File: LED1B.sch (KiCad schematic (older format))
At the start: 18 parts

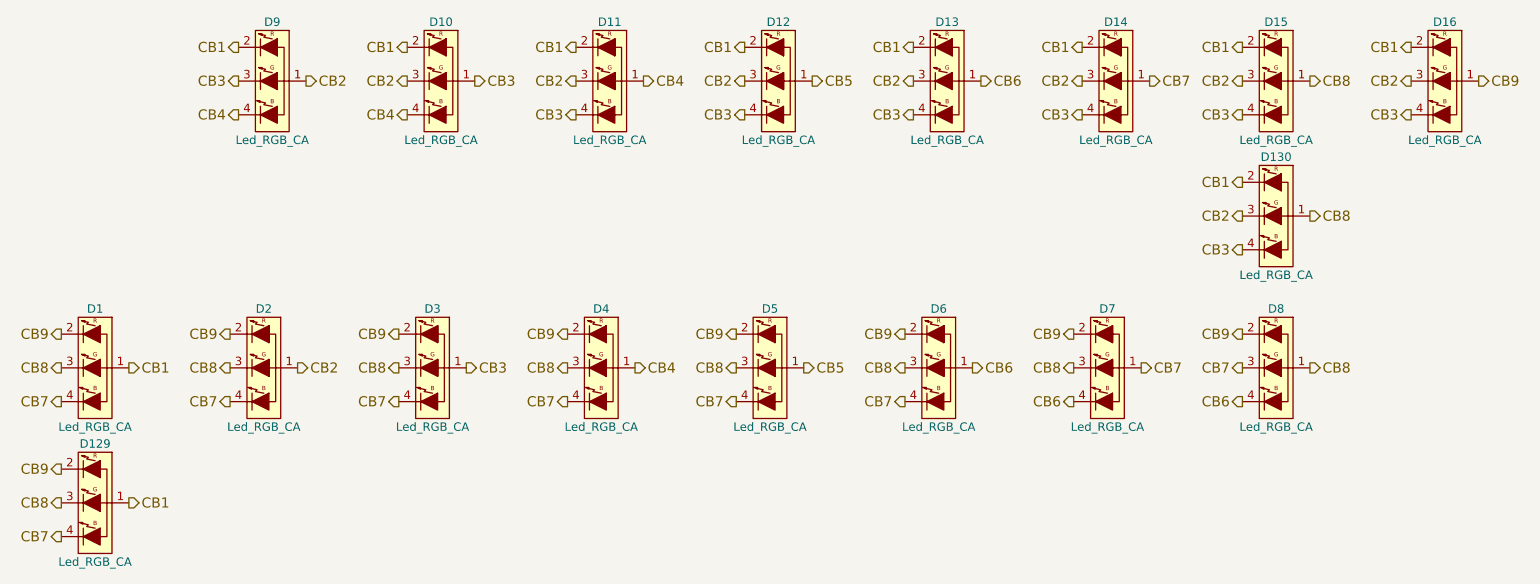
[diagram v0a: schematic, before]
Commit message: Did some visual cleanup.
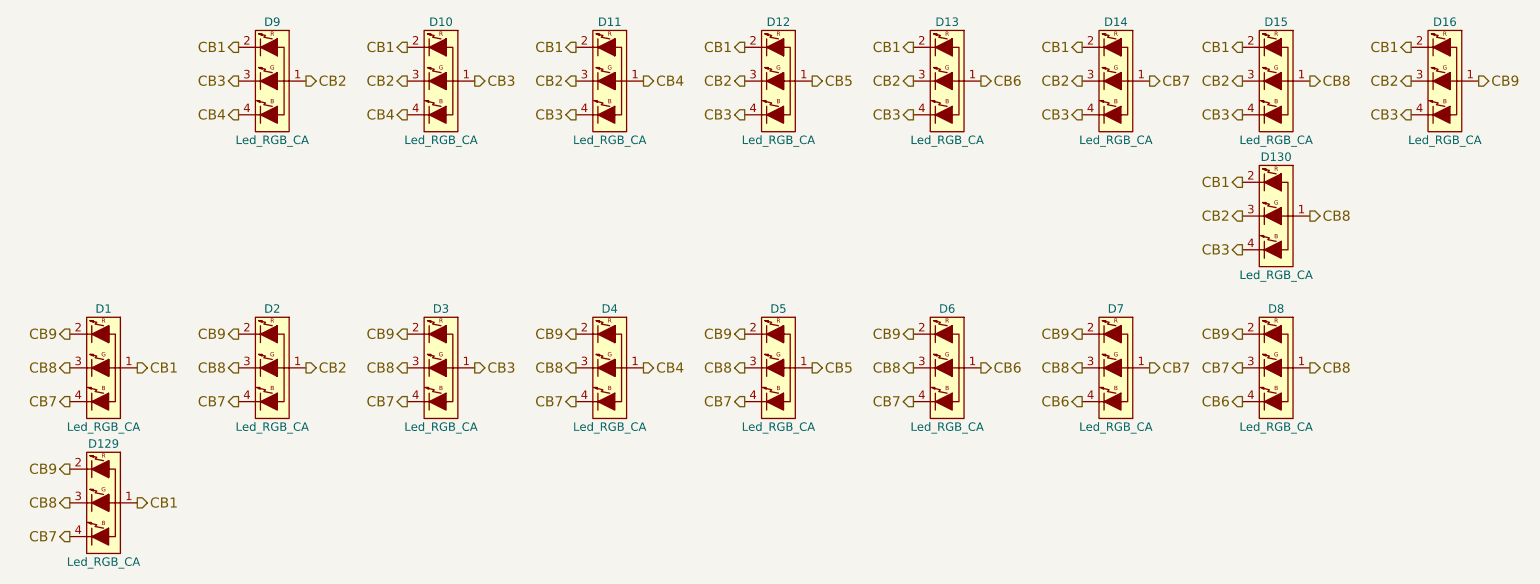
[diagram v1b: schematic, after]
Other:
- moved on the sheet: D1, D129, D2, D3, D4, D5, D6, D7
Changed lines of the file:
@@
 $Descr A4 11693 8268
 encoding utf-8
-Sheet 2 6
+Sheet 4 6
 Title ""
 Date ""
@@
 L Led_RGB_CA D1
 U 1 1 56C0E01C
-P 1950 3450
-F 0 "D1" H 1950 3800 50  0000 C CNN
-F 1 "Led_RGB_CA" H 1950 3100 50  0000 C CNN
-F 2 "mx2a:RGB" H 1905 3400 50  0001 C CNN
-F 3 "" H 1905 3400 50  0000 C CNN
-	1    1950 3450
+P 2000 3450
+F 0 "D1" H 2000 3800 50  0000 C CNN
+F 1 "Led_RGB_CA" H 2000 3100 50  0000 C CNN
+F 2 "mx2a:RGB" H 1955 3400 50  0001 C CNN
+F 3 "" H 1955 3400 50  0000 C CNN
+	1    2000 3450
 	1    0    0    -1
 $EndComp
@@
 L Led_RGB_CA D2
 U 1 1 56C0EC82
-P 2950 3450
-F 0 "D2" H 2950 3800 50  0000 C CNN
-F 1 "Led_RGB_CA" H 2950 3100 50  0000 C CNN
-F 2 "mx2a:RGB" H 2905 3400 50  0001 C CNN
-F 3 "" H 2905 3400 50  0000 C CNN
-	1    2950 3450
+P 3000 3450
+F 0 "D2" H 3000 3800 50  0000 C CNN
+F 1 "Led_RGB_CA" H 3000 3100 50  0000 C CNN
+F 2 "mx2a:RGB" H 2955 3400 50  0001 C CNN
+F 3 "" H 2955 3400 50  0000 C CNN
+	1    3000 3450
 	1    0    0    -1
 $EndComp
@@
 L Led_RGB_CA D3
 U 1 1 56C0F4C6
-P 3950 3450
-F 0 "D3" H 3950 3800 50  0000 C CNN
-F 1 "Led_RGB_CA" H 3950 3100 50  0000 C CNN
-F 2 "mx2a:RGB" H 3905 3400 50  0001 C CNN
-F 3 "" H 3905 3400 50  0000 C CNN
-	1    3950 3450
+P 4000 3450
+F 0 "D3" H 4000 3800 50  0000 C CNN
+F 1 "Led_RGB_CA" H 4000 3100 50  0000 C CNN
+F 2 "mx2a:RGB" H 3955 3400 50  0001 C CNN
+F 3 "" H 3955 3400 50  0000 C CNN
+	1    4000 3450
 	1    0    0    -1
 $EndComp
@@
 L Led_RGB_CA D4
 U 1 1 56C1065D
-P 4950 3450
-F 0 "D4" H 4950 3800 50  0000 C CNN
-F 1 "Led_RGB_CA" H 4950 3100 50  0000 C CNN
-F 2 "mx2a:RGB" H 4905 3400 50  0001 C CNN
-F 3 "" H 4905 3400 50  0000 C CNN
-	1    4950 3450
+P 5000 3450
+F 0 "D4" H 5000 3800 50  0000 C CNN
+F 1 "Led_RGB_CA" H 5000 3100 50  0000 C CNN
+F 2 "mx2a:RGB" H 4955 3400 50  0001 C CNN
+F 3 "" H 4955 3400 50  0000 C CNN
+	1    5000 3450
 	1    0    0    -1
 $EndComp
@@
 L Led_RGB_CA D5
 U 1 1 56C11695
-P 5950 3450
-F 0 "D5" H 5950 3800 50  0000 C CNN
-F 1 "Led_RGB_CA" H 5950 3100 50  0000 C CNN
-F 2 "mx2a:RGB" H 5905 3400 50  0001 C CNN
-F 3 "" H 5905 3400 50  0000 C CNN
-	1    5950 3450
+P 6000 3450
+F 0 "D5" H 6000 3800 50  0000 C CNN
+F 1 "Led_RGB_CA" H 6000 3100 50  0000 C CNN
+F 2 "mx2a:RGB" H 5955 3400 50  0001 C CNN
+F 3 "" H 5955 3400 50  0000 C CNN
+	1    6000 3450
 	1    0    0    -1
 $EndComp
@@
 L Led_RGB_CA D6
 U 1 1 56C12C27
-P 6950 3450
-F 0 "D6" H 6950 3800 50  0000 C CNN
-F 1 "Led_RGB_CA" H 6950 3100 50  0000 C CNN
-F 2 "mx2a:RGB" H 6905 3400 50  0001 C CNN
-F 3 "" H 6905 3400 50  0000 C CNN
-	1    6950 3450
+P 7000 3450
+F 0 "D6" H 7000 3800 50  0000 C CNN
+F 1 "Led_RGB_CA" H 7000 3100 50  0000 C CNN
+F 2 "mx2a:RGB" H 6955 3400 50  0001 C CNN
+F 3 "" H 6955 3400 50  0000 C CNN
+	1    7000 3450
 	1    0    0    -1
 $EndComp
@@
 L Led_RGB_CA D7
 U 1 1 56C14361
-P 7950 3450
-F 0 "D7" H 7950 3800 50  0000 C CNN
-F 1 "Led_RGB_CA" H 7950 3100 50  0000 C CNN
-F 2 "mx2a:RGB" H 7905 3400 50  0001 C CNN
-F 3 "" H 7905 3400 50  0000 C CNN
-	1    7950 3450
+P 8000 3450
+F 0 "D7" H 8000 3800 50  0000 C CNN
+F 1 "Led_RGB_CA" H 8000 3100 50  0000 C CNN
+F 2 "mx2a:RGB" H 7955 3400 50  0001 C CNN
+F 3 "" H 7955 3400 50  0000 C CNN
+	1    8000 3450
 	1    0    0    -1
 $EndComp
@@
 L Led_RGB_CA D129
 U 1 1 56EDAD96
-P 1950 4250
-F 0 "D129" H 1950 4600 50  0000 C CNN
-F 1 "Led_RGB_CA" H 1950 3900 50  0000 C CNN
-F 2 "mx2a:RGB" H 1905 4200 50  0001 C CNN
-F 3 "" H 1905 4200 50  0000 C CNN
-	1    1950 4250
+P 2000 4250
+F 0 "D129" H 2000 4600 50  0000 C CNN
+F 1 "Led_RGB_CA" H 2000 3900 50  0000 C CNN
+F 2 "mx2a:RGB" H 1955 4200 50  0001 C CNN
+F 3 "" H 1955 4200 50  0000 C CNN
+	1    2000 4250
 	1    0    0    -1
 $EndComp
@@
 Text HLabel 9750 1550 0    60   Output ~ 0
 CB1
-Text HLabel 2150 3450 2    60   Output ~ 0
-CB1
-Text HLabel 2150 4250 2    60   Output ~ 0
-CB1
-Text HLabel 1750 3650 0    60   Output ~ 0
-CB7
-Text HLabel 1750 4450 0    60   Output ~ 0
-CB7
-Text HLabel 1750 3450 0    60   Output ~ 0
-CB8
-Text HLabel 1750 4250 0    60   Output ~ 0
-CB8
-Text HLabel 1750 4050 0    60   Output ~ 0
-CB9
-Text HLabel 1750 3250 0    60   Output ~ 0
-CB9
-Text HLabel 2750 3650 0    60   Output ~ 0
-CB7
-Text HLabel 2750 3450 0    60   Output ~ 0
-CB8
-Text HLabel 2750 3250 0    60   Output ~ 0
-CB9
-Text HLabel 3150 3450 2    60   Output ~ 0
-CB2
-Text HLabel 3750 3650 0    60   Output ~ 0
-CB7
-Text HLabel 3750 3450 0    60   Output ~ 0
-CB8
-Text HLabel 3750 3250 0    60   Output ~ 0
-CB9
-Text HLabel 4150 3450 2    60   Output ~ 0
-CB3
-Text HLabel 4750 3650 0    60   Output ~ 0
-CB7
-Text HLabel 4750 3450 0    60   Output ~ 0
-CB8
-Text HLabel 4750 3250 0    60   Output ~ 0
-CB9
-Text HLabel 5150 3450 2    60   Output ~ 0
+Text HLabel 2200 3450 2    60   Output ~ 0
+CB1
+Text HLabel 2200 4250 2    60   Output ~ 0
+CB1
+Text HLabel 1800 3650 0    60   Output ~ 0
+CB7
+Text HLabel 1800 4450 0    60   Output ~ 0
+CB7
+Text HLabel 1800 3450 0    60   Output ~ 0
+CB8
+Text HLabel 1800 4250 0    60   Output ~ 0
+CB8
+Text HLabel 1800 4050 0    60   Output ~ 0
+CB9
+Text HLabel 1800 3250 0    60   Output ~ 0
+CB9
+Text HLabel 2800 3650 0    60   Output ~ 0
+CB7
+Text HLabel 2800 3450 0    60   Output ~ 0
+CB8
+Text HLabel 2800 3250 0    60   Output ~ 0
+CB9
+Text HLabel 3200 3450 2    60   Output ~ 0
+CB2
+Text HLabel 3800 3650 0    60   Output ~ 0
+CB7
+Text HLabel 3800 3450 0    60   Output ~ 0
+CB8
+Text HLabel 3800 3250 0    60   Output ~ 0
+CB9
+Text HLabel 4200 3450 2    60   Output ~ 0
+CB3
+Text HLabel 4800 3650 0    60   Output ~ 0
+CB7
+Text HLabel 4800 3450 0    60   Output ~ 0
+CB8
+Text HLabel 4800 3250 0    60   Output ~ 0
+CB9
+Text HLabel 5200 3450 2    60   Output ~ 0
 CB4
-Text HLabel 5750 3650 0    60   Output ~ 0
-CB7
-Text HLabel 5750 3450 0    60   Output ~ 0
-CB8
-Text HLabel 5750 3250 0    60   Output ~ 0
-CB9
-Text HLabel 6150 3450 2    60   Output ~ 0
+Text HLabel 5800 3650 0    60   Output ~ 0
+CB7
+Text HLabel 5800 3450 0    60   Output ~ 0
+CB8
+Text HLabel 5800 3250 0    60   Output ~ 0
+CB9
+Text HLabel 6200 3450 2    60   Output ~ 0
 CB5
-Text HLabel 6750 3650 0    60   Output ~ 0
-CB7
-Text HLabel 6750 3450 0    60   Output ~ 0
-CB8
-Text HLabel 6750 3250 0    60   Output ~ 0
-CB9
-Text HLabel 7150 3450 2    60   Output ~ 0
+Text HLabel 6800 3650 0    60   Output ~ 0
+CB7
+Text HLabel 6800 3450 0    60   Output ~ 0
+CB8
+Text HLabel 6800 3250 0    60   Output ~ 0
+CB9
+Text HLabel 7200 3450 2    60   Output ~ 0
 CB6
-Text HLabel 8150 3450 2    60   Output ~ 0
-CB7
-Text HLabel 7750 3450 0    60   Output ~ 0
-CB8
-Text HLabel 7750 3250 0    60   Output ~ 0
-CB9
-Text HLabel 7750 3650 0    60   Output ~ 0
+Text HLabel 8200 3450 2    60   Output ~ 0
+CB7
+Text HLabel 7800 3450 0    60   Output ~ 0
+CB8
+Text HLabel 7800 3250 0    60   Output ~ 0
+CB9
+Text HLabel 7800 3650 0    60   Output ~ 0
 CB6
 Text HLabel 8750 3250 0    60   Output ~ 0

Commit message: Switched to a different USB Port and 100uF Cap
also added a USB-Debug Header and did some cleanup
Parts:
- D1, D10, D11, D12, D129, D13, D130, D14, D15, D16, D2, D3, D4, D5, D6, D7, D8, D9: footprint mx2a:RGB -> libs.pretty:RGB
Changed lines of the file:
@@
 U 1 1 56C094FB
 P 3000 1750
+AR Path="/56C094FB" Ref="D9"  Part="1"
+AR Path="/576308BB/56C094FB" Ref="D9"  Part="1"
 F 0 "D9" H 3000 2100 50  0000 C CNN
 F 1 "Led_RGB_CA" H 3000 1400 50  0000 C CNN
-F 2 "mx2a:RGB" H 2955 1700 50  0001 C CNN
+F 2 "libs.pretty:RGB" H 2955 1700 50  0001 C CNN
 F 3 "" H 2955 1700 50  0000 C CNN
 	1    3000 1750
@@
 U 1 1 56C0963F
 P 4000 1750
+AR Path="/56C0963F" Ref="D10"  Part="1"
+AR Path="/576308BB/56C0963F" Ref="D10"  Part="1"
 F 0 "D10" H 4000 2100 50  0000 C CNN
 F 1 "Led_RGB_CA" H 4000 1400 50  0000 C CNN
-F 2 "mx2a:RGB" H 3955 1700 50  0001 C CNN
+F 2 "libs.pretty:RGB" H 3955 1700 50  0001 C CNN
 F 3 "" H 3955 1700 50  0000 C CNN
 	1    4000 1750
@@
 U 1 1 56C098D4
 P 5000 1750
+AR Path="/56C098D4" Ref="D11"  Part="1"
+AR Path="/576308BB/56C098D4" Ref="D11"  Part="1"
 F 0 "D11" H 5000 2100 50  0000 C CNN
 F 1 "Led_RGB_CA" H 5000 1400 50  0000 C CNN
-F 2 "mx2a:RGB" H 4955 1700 50  0001 C CNN
+F 2 "libs.pretty:RGB" H 4955 1700 50  0001 C CNN
 F 3 "" H 4955 1700 50  0000 C CNN
 	1    5000 1750
@@
 U 1 1 56C0A50A
 P 6000 1750
+AR Path="/56C0A50A" Ref="D12"  Part="1"
+AR Path="/576308BB/56C0A50A" Ref="D12"  Part="1"
 F 0 "D12" H 6000 2100 50  0000 C CNN
 F 1 "Led_RGB_CA" H 6000 1400 50  0000 C CNN
-F 2 "mx2a:RGB" H 5955 1700 50  0001 C CNN
+F 2 "libs.pretty:RGB" H 5955 1700 50  0001 C CNN
 F 3 "" H 5955 1700 50  0000 C CNN
 	1    6000 1750
@@
 U 1 1 56C0AF61
 P 7000 1750
+AR Path="/56C0AF61" Ref="D13"  Part="1"
+AR Path="/576308BB/56C0AF61" Ref="D13"  Part="1"
 F 0 "D13" H 7000 2100 50  0000 C CNN
 F 1 "Led_RGB_CA" H 7000 1400 50  0000 C CNN
-F 2 "mx2a:RGB" H 6955 1700 50  0001 C CNN
+F 2 "libs.pretty:RGB" H 6955 1700 50  0001 C CNN
 F 3 "" H 6955 1700 50  0000 C CNN
 	1    7000 1750
@@
 U 1 1 56C0B3C7
 P 8000 1750
+AR Path="/56C0B3C7" Ref="D14"  Part="1"
+AR Path="/576308BB/56C0B3C7" Ref="D14"  Part="1"
 F 0 "D14" H 8000 2100 50  0000 C CNN
 F 1 "Led_RGB_CA" H 8000 1400 50  0000 C CNN
-F 2 "mx2a:RGB" H 7955 1700 50  0001 C CNN
+F 2 "libs.pretty:RGB" H 7955 1700 50  0001 C CNN
 F 3 "" H 7955 1700 50  0000 C CNN
 	1    8000 1750
@@
 U 1 1 56C0C0F2
 P 8950 1750
+AR Path="/56C0C0F2" Ref="D15"  Part="1"
+AR Path="/576308BB/56C0C0F2" Ref="D15"  Part="1"
 F 0 "D15" H 8950 2100 50  0000 C CNN
 F 1 "Led_RGB_CA" H 8950 1400 50  0000 C CNN
-F 2 "mx2a:RGB" H 8905 1700 50  0001 C CNN
+F 2 "libs.pretty:RGB" H 8905 1700 50  0001 C CNN
 F 3 "" H 8905 1700 50  0000 C CNN
 	1    8950 1750
@@
 U 1 1 56C0D59D
 P 9950 1750
+AR Path="/56C0D59D" Ref="D16"  Part="1"
+AR Path="/576308BB/56C0D59D" Ref="D16"  Part="1"
 F 0 "D16" H 9950 2100 50  0000 C CNN
 F 1 "Led_RGB_CA" H 9950 1400 50  0000 C CNN
-F 2 "mx2a:RGB" H 9905 1700 50  0001 C CNN
+F 2 "libs.pretty:RGB" H 9905 1700 50  0001 C CNN
 F 3 "" H 9905 1700 50  0000 C CNN
 	1    9950 1750
@@
 U 1 1 56C0E01C
 P 2000 3450
+AR Path="/56C0E01C" Ref="D1"  Part="1"
+AR Path="/576308BB/56C0E01C" Ref="D1"  Part="1"
 F 0 "D1" H 2000 3800 50  0000 C CNN
 F 1 "Led_RGB_CA" H 2000 3100 50  0000 C CNN
-F 2 "mx2a:RGB" H 1955 3400 50  0001 C CNN
+F 2 "libs.pretty:RGB" H 1955 3400 50  0001 C CNN
 F 3 "" H 1955 3400 50  0000 C CNN
 	1    2000 3450
@@
 U 1 1 56C0EC82
 P 3000 3450
+AR Path="/56C0EC82" Ref="D2"  Part="1"
+AR Path="/576308BB/56C0EC82" Ref="D2"  Part="1"
 F 0 "D2" H 3000 3800 50  0000 C CNN
 F 1 "Led_RGB_CA" H 3000 3100 50  0000 C CNN
-F 2 "mx2a:RGB" H 2955 3400 50  0001 C CNN
+F 2 "libs.pretty:RGB" H 2955 3400 50  0001 C CNN
 F 3 "" H 2955 3400 50  0000 C CNN
 	1    3000 3450
@@
 U 1 1 56C0F4C6
 P 4000 3450
+AR Path="/56C0F4C6" Ref="D3"  Part="1"
+AR Path="/576308BB/56C0F4C6" Ref="D3"  Part="1"
 F 0 "D3" H 4000 3800 50  0000 C CNN
 F 1 "Led_RGB_CA" H 4000 3100 50  0000 C CNN
-F 2 "mx2a:RGB" H 3955 3400 50  0001 C CNN
+F 2 "libs.pretty:RGB" H 3955 3400 50  0001 C CNN
 F 3 "" H 3955 3400 50  0000 C CNN
 	1    4000 3450
@@
 U 1 1 56C1065D
 P 5000 3450
+AR Path="/56C1065D" Ref="D4"  Part="1"
+AR Path="/576308BB/56C1065D" Ref="D4"  Part="1"
 F 0 "D4" H 5000 3800 50  0000 C CNN
 F 1 "Led_RGB_CA" H 5000 3100 50  0000 C CNN
-F 2 "mx2a:RGB" H 4955 3400 50  0001 C CNN
+F 2 "libs.pretty:RGB" H 4955 3400 50  0001 C CNN
 F 3 "" H 4955 3400 50  0000 C CNN
 	1    5000 3450
@@
 U 1 1 56C11695
 P 6000 3450
+AR Path="/56C11695" Ref="D5"  Part="1"
+AR Path="/576308BB/56C11695" Ref="D5"  Part="1"
 F 0 "D5" H 6000 3800 50  0000 C CNN
 F 1 "Led_RGB_CA" H 6000 3100 50  0000 C CNN
-F 2 "mx2a:RGB" H 5955 3400 50  0001 C CNN
+F 2 "libs.pretty:RGB" H 5955 3400 50  0001 C CNN
 F 3 "" H 5955 3400 50  0000 C CNN
 	1    6000 3450
@@
 U 1 1 56C12C27
 P 7000 3450
+AR Path="/56C12C27" Ref="D6"  Part="1"
+AR Path="/576308BB/56C12C27" Ref="D6"  Part="1"
 F 0 "D6" H 7000 3800 50  0000 C CNN
 F 1 "Led_RGB_CA" H 7000 3100 50  0000 C CNN
-F 2 "mx2a:RGB" H 6955 3400 50  0001 C CNN
+F 2 "libs.pretty:RGB" H 6955 3400 50  0001 C CNN
 F 3 "" H 6955 3400 50  0000 C CNN
 	1    7000 3450
@@
 U 1 1 56C14361
 P 8000 3450
+AR Path="/56C14361" Ref="D7"  Part="1"
+AR Path="/576308BB/56C14361" Ref="D7"  Part="1"
 F 0 "D7" H 8000 3800 50  0000 C CNN
 F 1 "Led_RGB_CA" H 8000 3100 50  0000 C CNN
-F 2 "mx2a:RGB" H 7955 3400 50  0001 C CNN
+F 2 "libs.pretty:RGB" H 7955 3400 50  0001 C CNN
 F 3 "" H 7955 3400 50  0000 C CNN
 	1    8000 3450
@@
 U 1 1 56C143BE
 P 8950 3450
+AR Path="/56C143BE" Ref="D8"  Part="1"
+AR Path="/576308BB/56C143BE" Ref="D8"  Part="1"
 F 0 "D8" H 8950 3800 50  0000 C CNN
 F 1 "Led_RGB_CA" H 8950 3100 50  0000 C CNN
-F 2 "mx2a:RGB" H 8905 3400 50  0001 C CNN
+F 2 "libs.pretty:RGB" H 8905 3400 50  0001 C CNN
 F 3 "" H 8905 3400 50  0000 C CNN
 	1    8950 3450
@@
 U 1 1 56EDAD96
 P 2000 4250
+AR Path="/56EDAD96" Ref="D129"  Part="1"
+AR Path="/576308BB/56EDAD96" Ref="D129"  Part="1"
 F 0 "D129" H 2000 4600 50  0000 C CNN
 F 1 "Led_RGB_CA" H 2000 3900 50  0000 C CNN
-F 2 "mx2a:RGB" H 1955 4200 50  0001 C CNN
+F 2 "libs.pretty:RGB" H 1955 4200 50  0001 C CNN
 F 3 "" H 1955 4200 50  0000 C CNN
 	1    2000 4250
@@
 U 1 1 56EDB705
 P 8950 2550
+AR Path="/56EDB705" Ref="D130"  Part="1"
+AR Path="/576308BB/56EDB705" Ref="D130"  Part="1"
 F 0 "D130" H 8950 2900 50  0000 C CNN
 F 1 "Led_RGB_CA" H 8950 2200 50  0000 C CNN
-F 2 "mx2a:RGB" H 8905 2500 50  0001 C CNN
+F 2 "libs.pretty:RGB" H 8905 2500 50  0001 C CNN
 F 3 "" H 8905 2500 50  0000 C CNN
 	1    8950 2550
